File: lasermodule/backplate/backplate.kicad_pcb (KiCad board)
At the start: 2 copper layers, 33.2 x 64.1 mm, 6 parts, among them J1 Conn_01x01, J2 Conn_01x01, J3 Conn_01x01, J4 Conn_01x01

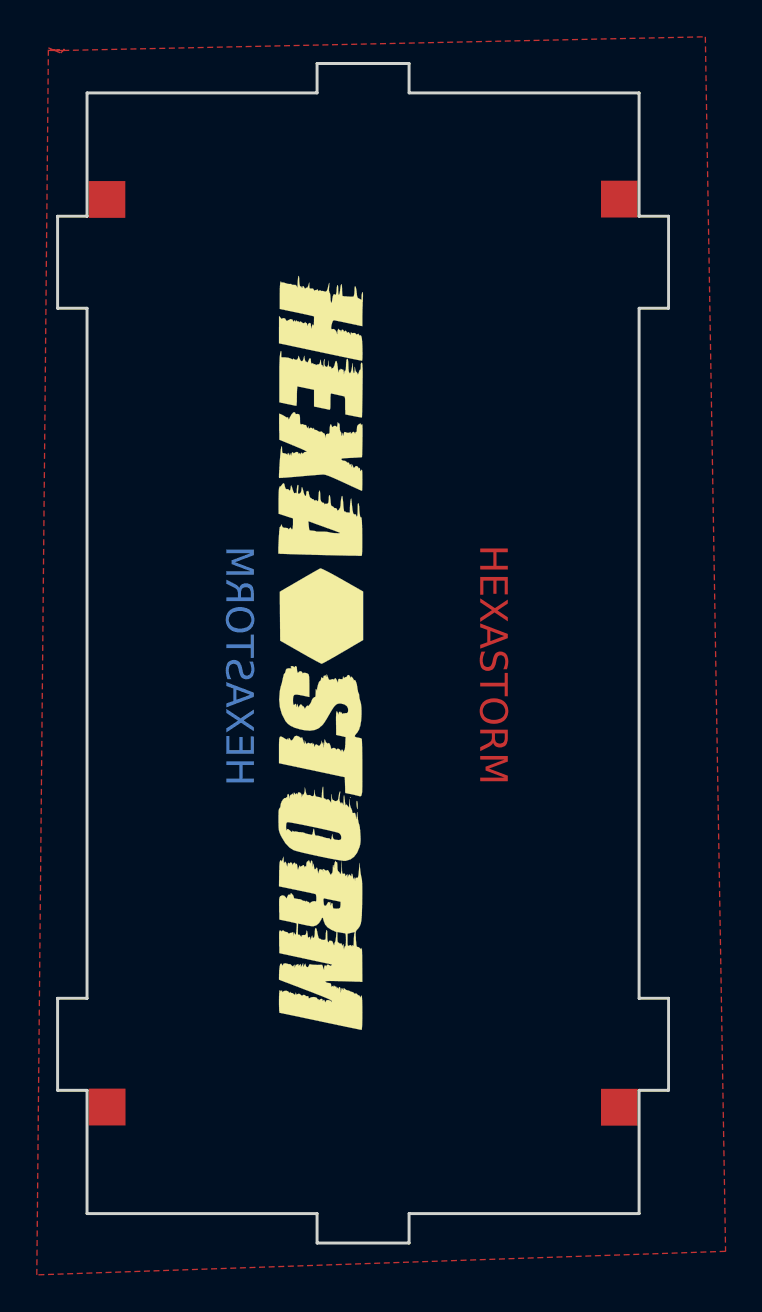
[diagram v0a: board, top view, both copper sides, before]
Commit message: board almost fully synced close for release
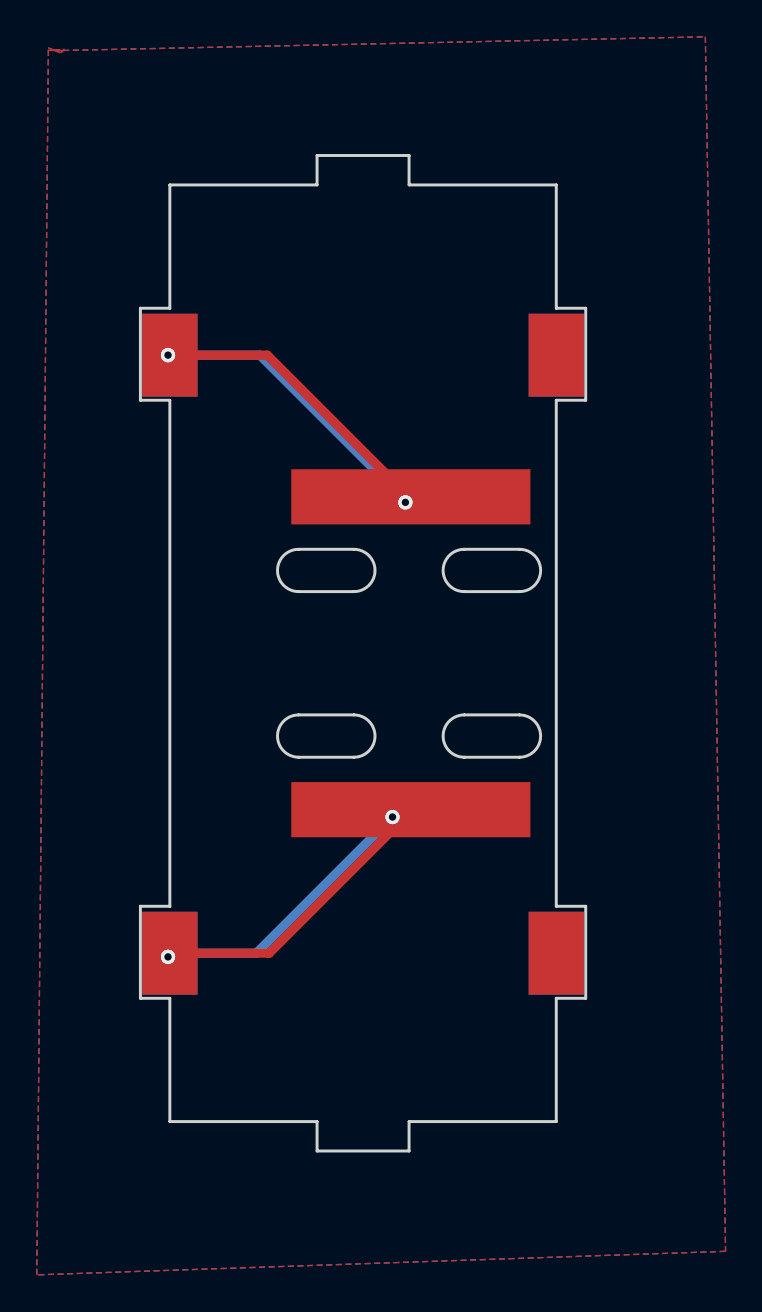
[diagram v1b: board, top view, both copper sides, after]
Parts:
- removed L1, L2: Logo_Open_Hardware_Large, footprints:hexastorm
- added J5: Conn_01x02, footprints:pogopincontact, F.Cu at (156.7, 103.9)
- moved J2 9.15 mm to (164.6, 87.7), turned to 90 degrees
- moved J1 9.13 mm to (143.6, 87.7), turned to 90 degrees
- moved J3 9.05 mm to (164.6, 120.2), turned to 90 degrees
- moved J4 9.03 mm to (143.6, 120.2), turned to -90 degrees
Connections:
- J1 pad 1: unconnected-(J1-Pin_1-Pad1) -> +12V
- J4 pad 1: unconnected-(J4-Pin_1-Pad1) -> LDK
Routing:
- net +12V: track 0.00 -> 32.6 mm, vias 0 -> 2
- net LDK: track 0.00 -> 31.9 mm, vias 0 -> 2
- added copper zone on B.Cu, net LDK
- added copper zone on F.Cu, net LDK
- removed copper zone on F.Cu, net (none)
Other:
- board size 33.2 x 64.1 mm -> 24.2 x 54.1 mm
- board text removed: "HEXASTORM"
